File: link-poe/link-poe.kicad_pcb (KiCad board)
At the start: 4 copper layers, 70 x 22 mm, 41 parts, among them J101 2x05_Horizontal, J102 NE8FAH, J103 JAE_DX07S016JA3, J104 2x05_Horizontal, J105 NE8FAH, J106 WAGO-2065, J107 WAGO-2065, J108 WAGO-2065, J109 WAGO-2065, Q301 BSC010N04LS, Q302 BSC010N04LS, U301 LM74502-Q1, U501 TPSM33625

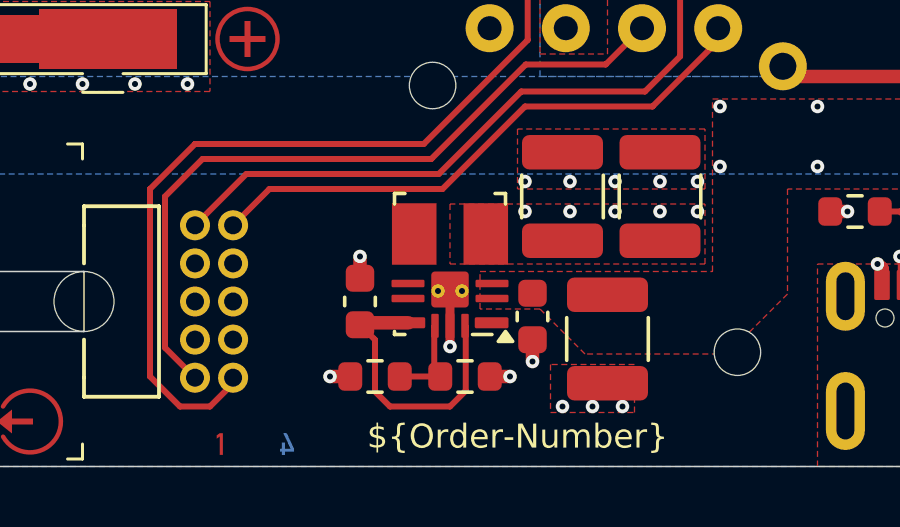
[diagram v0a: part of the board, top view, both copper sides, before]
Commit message: Refresh
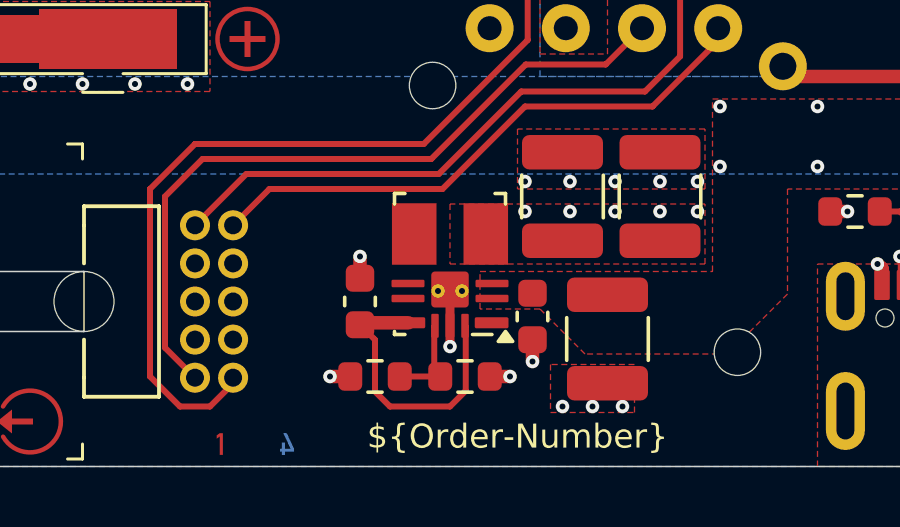
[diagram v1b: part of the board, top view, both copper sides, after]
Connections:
- net /+24V-Supply renamed /+24V-Link
